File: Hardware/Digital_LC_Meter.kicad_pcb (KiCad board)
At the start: 2 copper layers, 160 x 99.1 mm, 26 parts

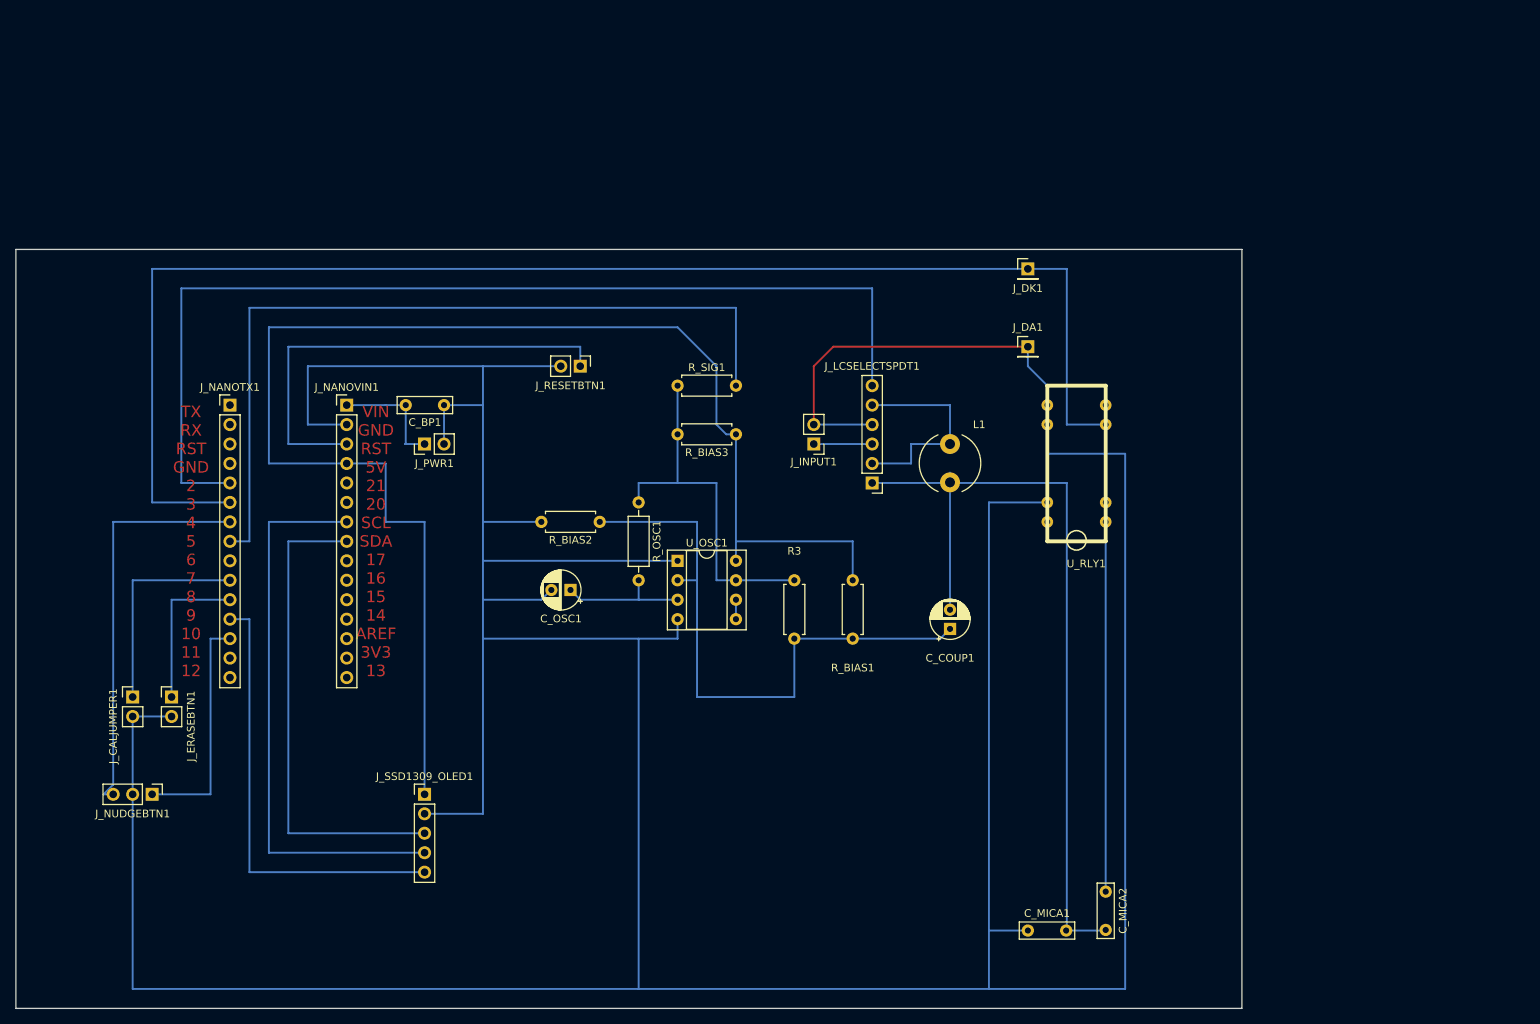
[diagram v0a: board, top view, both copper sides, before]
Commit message: updated docs
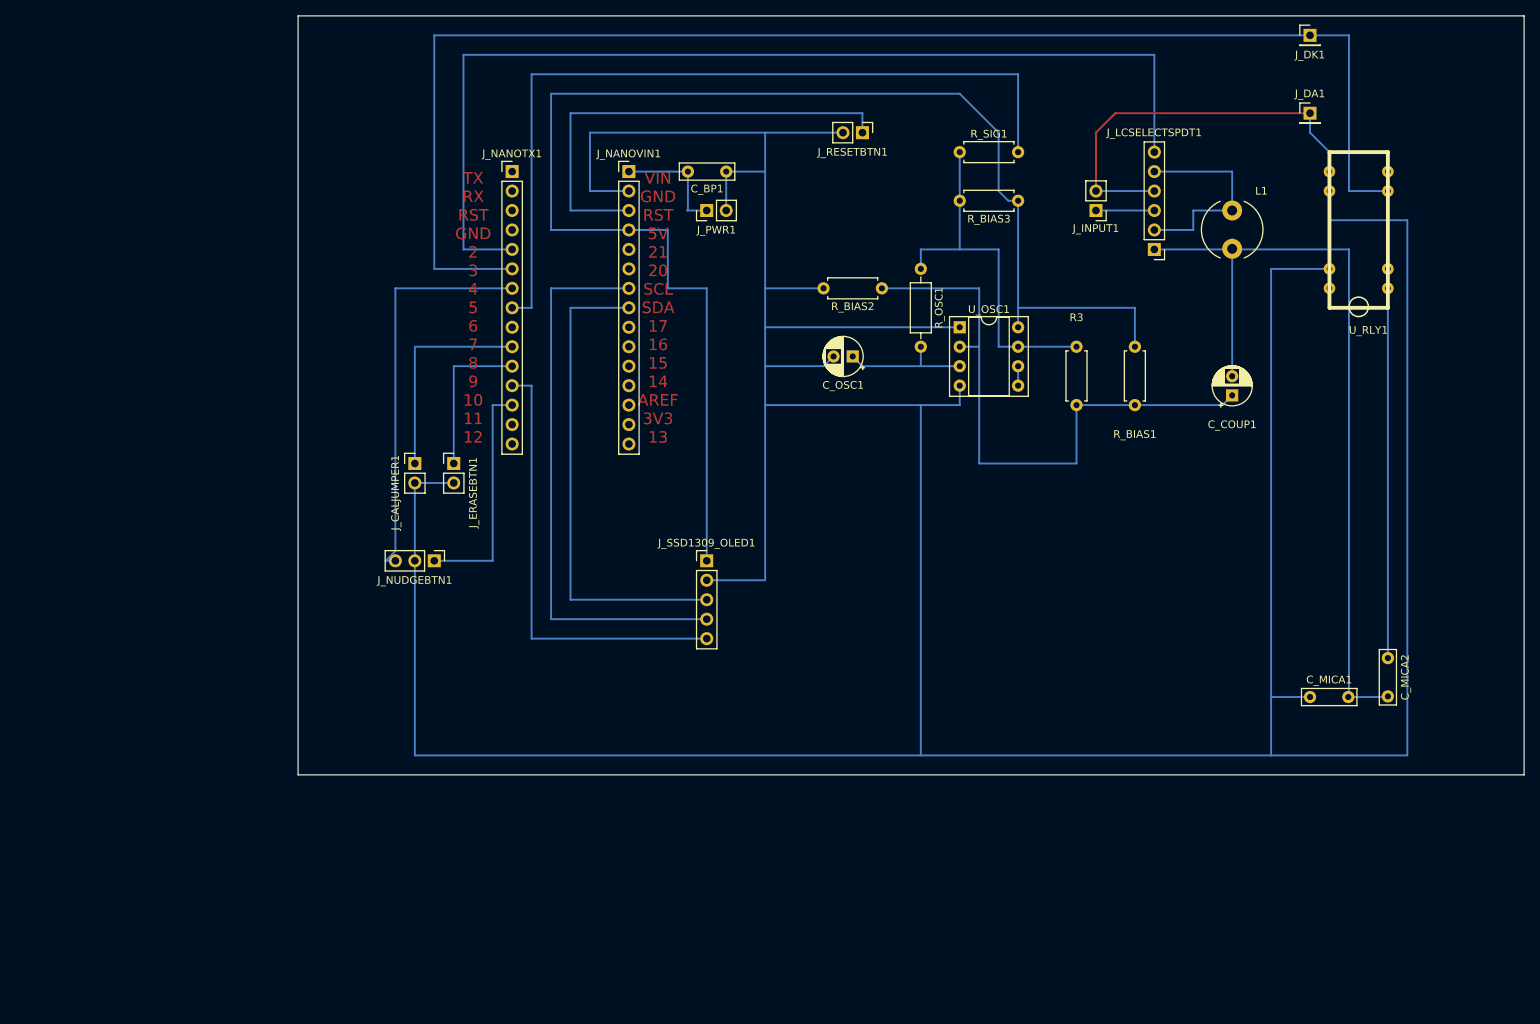
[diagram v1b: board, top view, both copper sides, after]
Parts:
- moved C_COUP1 47.8 mm to (184.2, 92.7)
- moved J_CALJUMPER1 47.8 mm to (77.5, 101.6)
- moved J_DK1 47.8 mm to (194.3, 45.7)
- moved J_ERASEBTN1 47.8 mm to (82.5, 101.6)
- moved J_INPUT1 47.8 mm to (166.4, 68.6)
- moved J_LCSELECTSPDT1 47.8 mm to (174.0, 73.7)
- moved L1 47.8 mm to (184.2, 68.6)
- moved R3 47.8 mm to (163.8, 86.4)
- moved R_BIAS2 47.8 mm to (138.4, 78.7)
- moved R_BIAS3 47.8 mm to (156.2, 67.3)
- moved C_BP1 47.8 mm to (118.1, 63.5)
- moved C_MICA1 47.8 mm to (194.3, 132.1)
- moved C_MICA2 47.8 mm to (204.5, 127.0)
- moved C_OSC1 47.8 mm to (134.6, 87.6)
- moved J_DA1 47.8 mm to (194.3, 55.9)
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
